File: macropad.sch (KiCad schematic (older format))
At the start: 13 parts

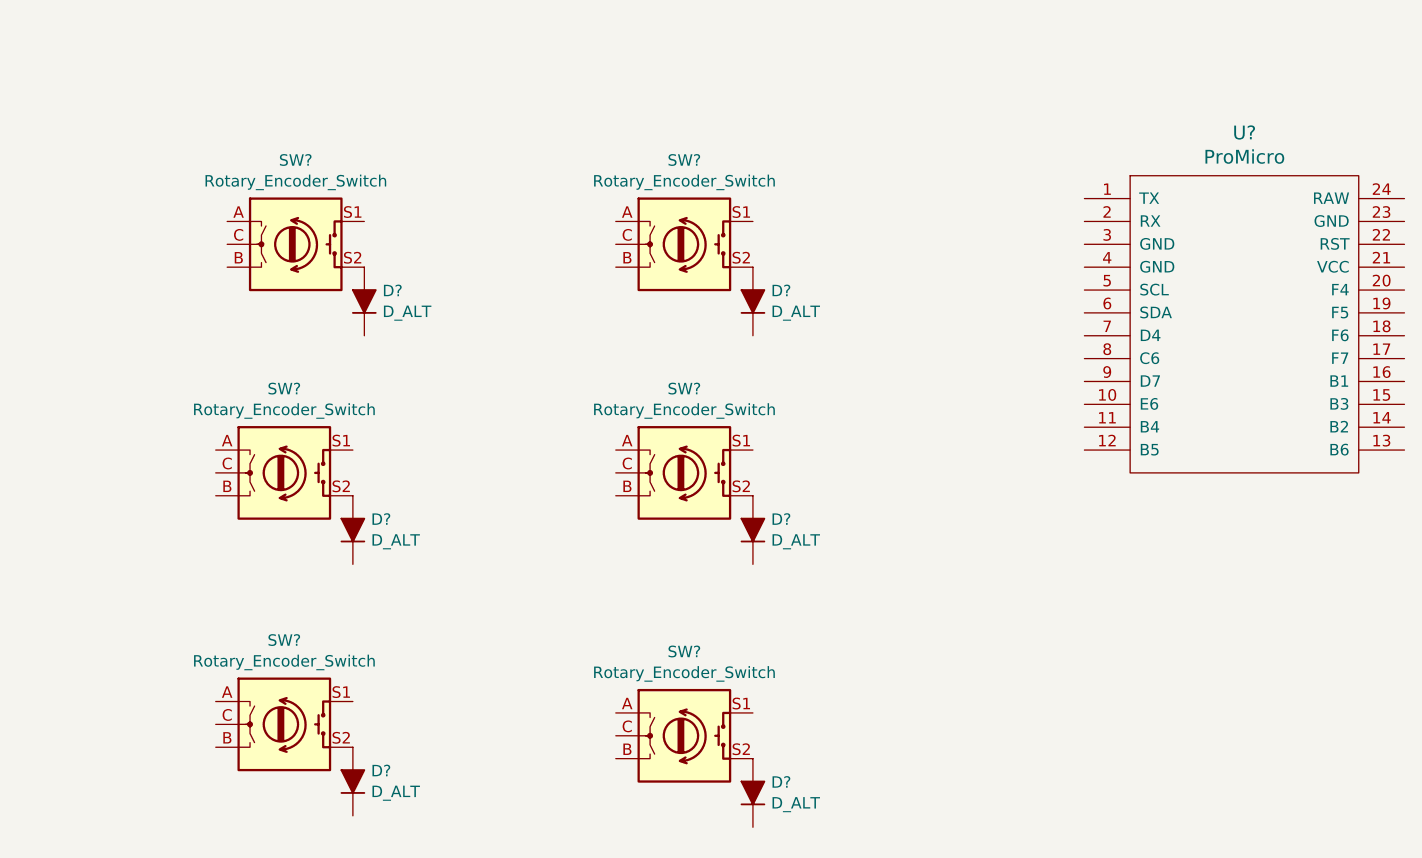
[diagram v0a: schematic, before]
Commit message: added some wires
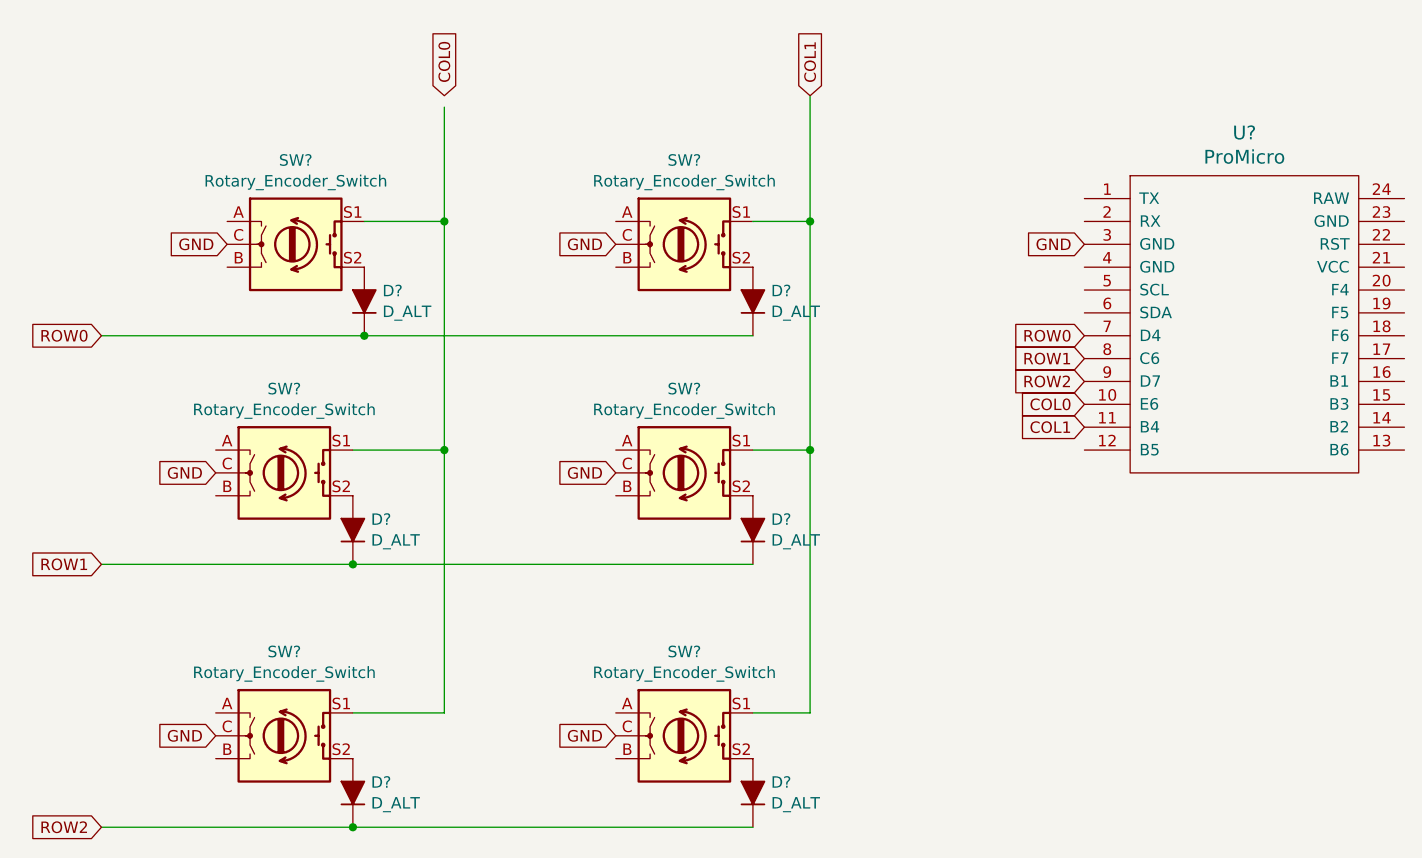
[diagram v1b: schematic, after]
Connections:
- net labels added: COL0, COL1, GND, ROW0, ROW1, ROW2
- wire segments 0 -> 18
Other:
- moved on the sheet: D?, SW?
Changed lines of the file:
@@
 L Device:Rotary_Encoder_Switch SW?
 U 1 1 5D79E7D6
-P 3600 4300
-F 0 "SW?" H 3600 4667 50  0000 C CNN
-F 1 "Rotary_Encoder_Switch" H 3600 4576 50  0000 C CNN
-F 2 "" H 3450 4460 50  0001 C CNN
-F 3 "~" H 3600 4560 50  0001 C CNN
-	1    3600 4300
+P 3600 4350
+F 0 "SW?" H 3600 4717 50  0000 C CNN
+F 1 "Rotary_Encoder_Switch" H 3600 4626 50  0000 C CNN
+F 2 "" H 3450 4510 50  0001 C CNN
+F 3 "~" H 3600 4610 50  0001 C CNN
+	1    3600 4350
 	1    0    0    -1
 $EndComp
@@
 L Device:D_ALT D?
 U 1 1 5D79F668
-P 3900 4550
-F 0 "D?" V 3946 4471 50  0000 R CNN
-F 1 "D_ALT" V 3855 4471 50  0000 R CNN
-F 2 "" H 3900 4550 50  0001 C CNN
-F 3 "~" H 3900 4550 50  0001 C CNN
-	1    3900 4550
+P 3900 4600
+F 0 "D?" V 3946 4521 50  0000 R CNN
+F 1 "D_ALT" V 3855 4521 50  0000 R CNN
+F 2 "" H 3900 4600 50  0001 C CNN
+F 3 "~" H 3900 4600 50  0001 C CNN
+	1    3900 4600
 	0    -1   -1   0
 $EndComp
@@
 	0    -1   -1   0
 $EndComp
+Wire Wire Line
+	3950 2100 4300 2100
+Wire Wire Line
+	4300 2100 4300 3100
+Wire Wire Line
+	4300 3100 3900 3100
+Wire Wire Line
+	3900 4250 4300 4250
+Wire Wire Line
+	4300 4250 4300 3100
+Connection ~ 4300 3100
+Wire Wire Line
+	4300 2100 4300 1600
+Connection ~ 4300 2100
+Text GLabel 4300 1550 1    50   Input ~ 0
+COL0
+Text GLabel 5900 1550 1    50   Input ~ 0
+COL1
+Wire Wire Line
+	5900 1550 5900 2100
+Wire Wire Line
+	5900 2100 5650 2100
+Wire Wire Line
+	5900 2100 5900 3100
+Wire Wire Line
+	5900 3100 5650 3100
+Connection ~ 5900 2100
+Wire Wire Line
+	5900 3100 5900 4250
+Wire Wire Line
+	5900 4250 5650 4250
+Connection ~ 5900 3100
+Wire Wire Line
+	5650 2600 3950 2600
+Connection ~ 3950 2600
+Wire Wire Line
+	3950 2600 2800 2600
+Wire Wire Line
+	5650 3600 3900 3600
+Connection ~ 3900 3600
+Wire Wire Line
+	3900 3600 2800 3600
+Wire Wire Line
+	5650 4750 3900 4750
+Connection ~ 3900 4750
+Wire Wire Line
+	3900 4750 2800 4750
+Text GLabel 2800 2600 0    50   Input ~ 0
+ROW0
+Text GLabel 2800 3600 0    50   Input ~ 0
+ROW1
+Text GLabel 2800 4750 0    50   Input ~ 0
+ROW2
+Text GLabel 3350 2200 0    50   Input ~ 0
+GND
+Text GLabel 3300 3200 0    50   Input ~ 0
+GND
+Text GLabel 3300 4350 0    50   Input ~ 0
+GND
+Text GLabel 5050 2200 0    50   Input ~ 0
+GND
+Text GLabel 5050 3200 0    50   Input ~ 0
+GND
+Text GLabel 5050 4350 0    50   Input ~ 0
+GND
+Text GLabel 7100 2200 0    50   Input ~ 0
+GND
+Text GLabel 7100 2600 0    50   Input ~ 0
+ROW0
+Text GLabel 7100 2700 0    50   Input ~ 0
+ROW1
+Text GLabel 7100 2800 0    50   Input ~ 0
+ROW2
+Text GLabel 7100 2900 0    50   Input ~ 0
+COL0
+Text GLabel 7100 3000 0    50   Input ~ 0
+COL1
 $EndSCHEMATC
